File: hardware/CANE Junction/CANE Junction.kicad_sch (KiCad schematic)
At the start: 20 parts, among them J101 Conn_02x05_Odd_Even, SW101 SW_Push, U1 MX25L3233FM2, U101 NCP163ASN330T1G, U102 NCP163ASN330T1G, U103 XMSM0G3507SDGS28R

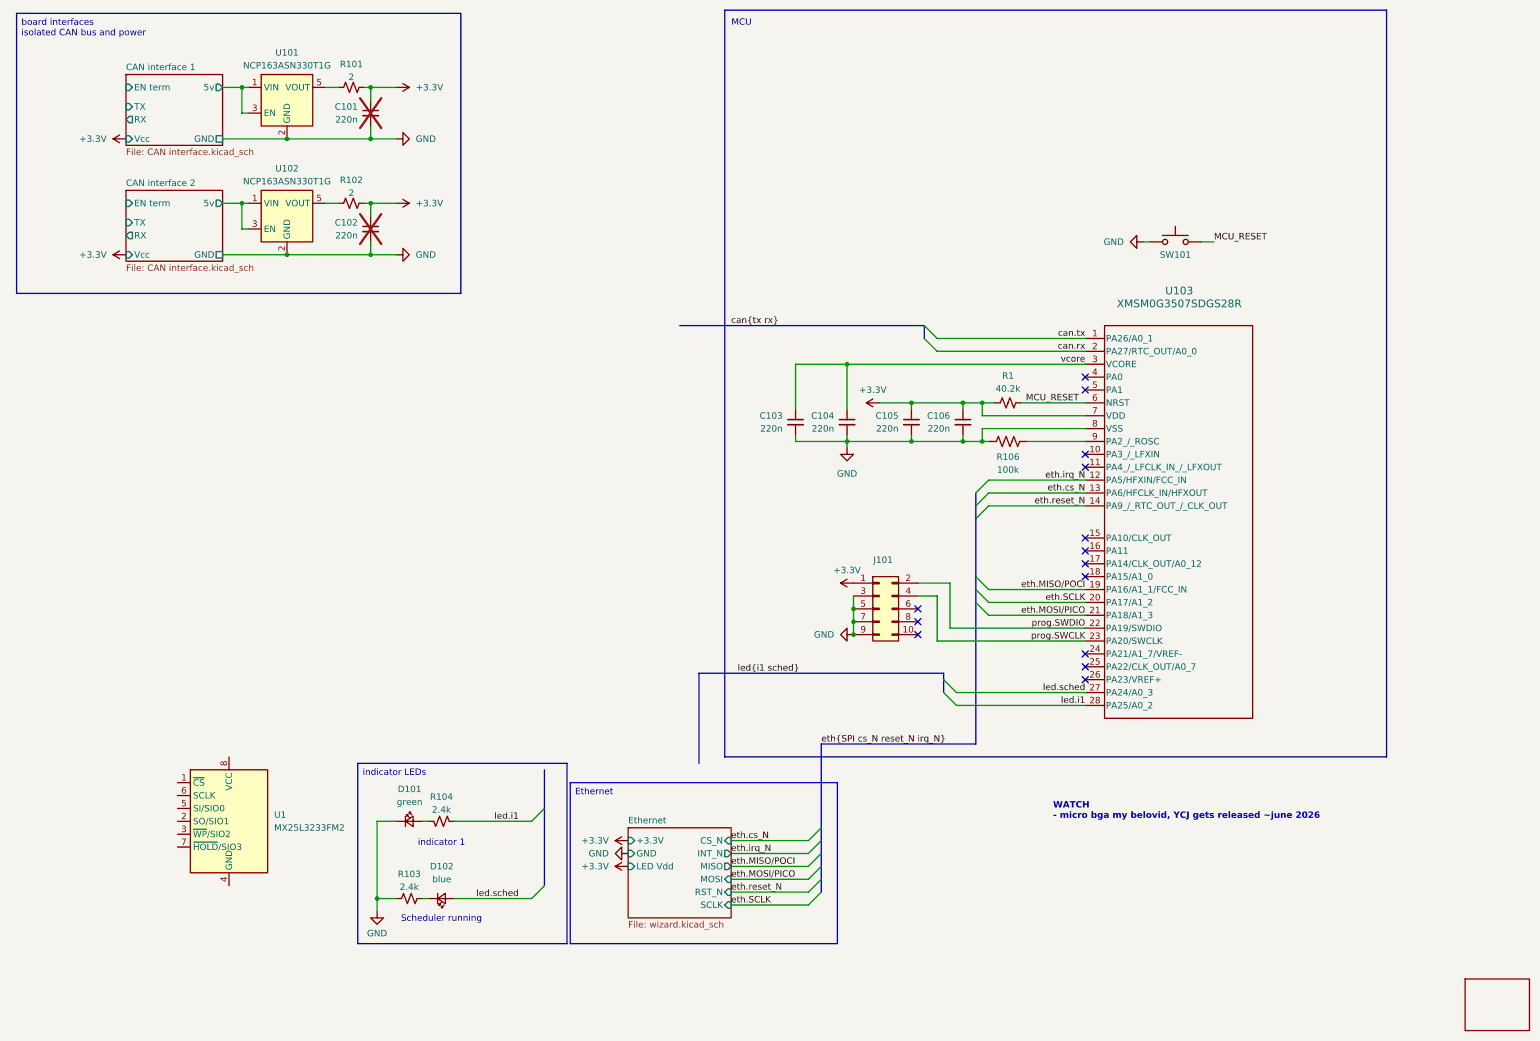
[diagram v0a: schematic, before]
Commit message: shuffle master 2000
nearing terminal shuffle . main components in, awaiting general and layout tie ins
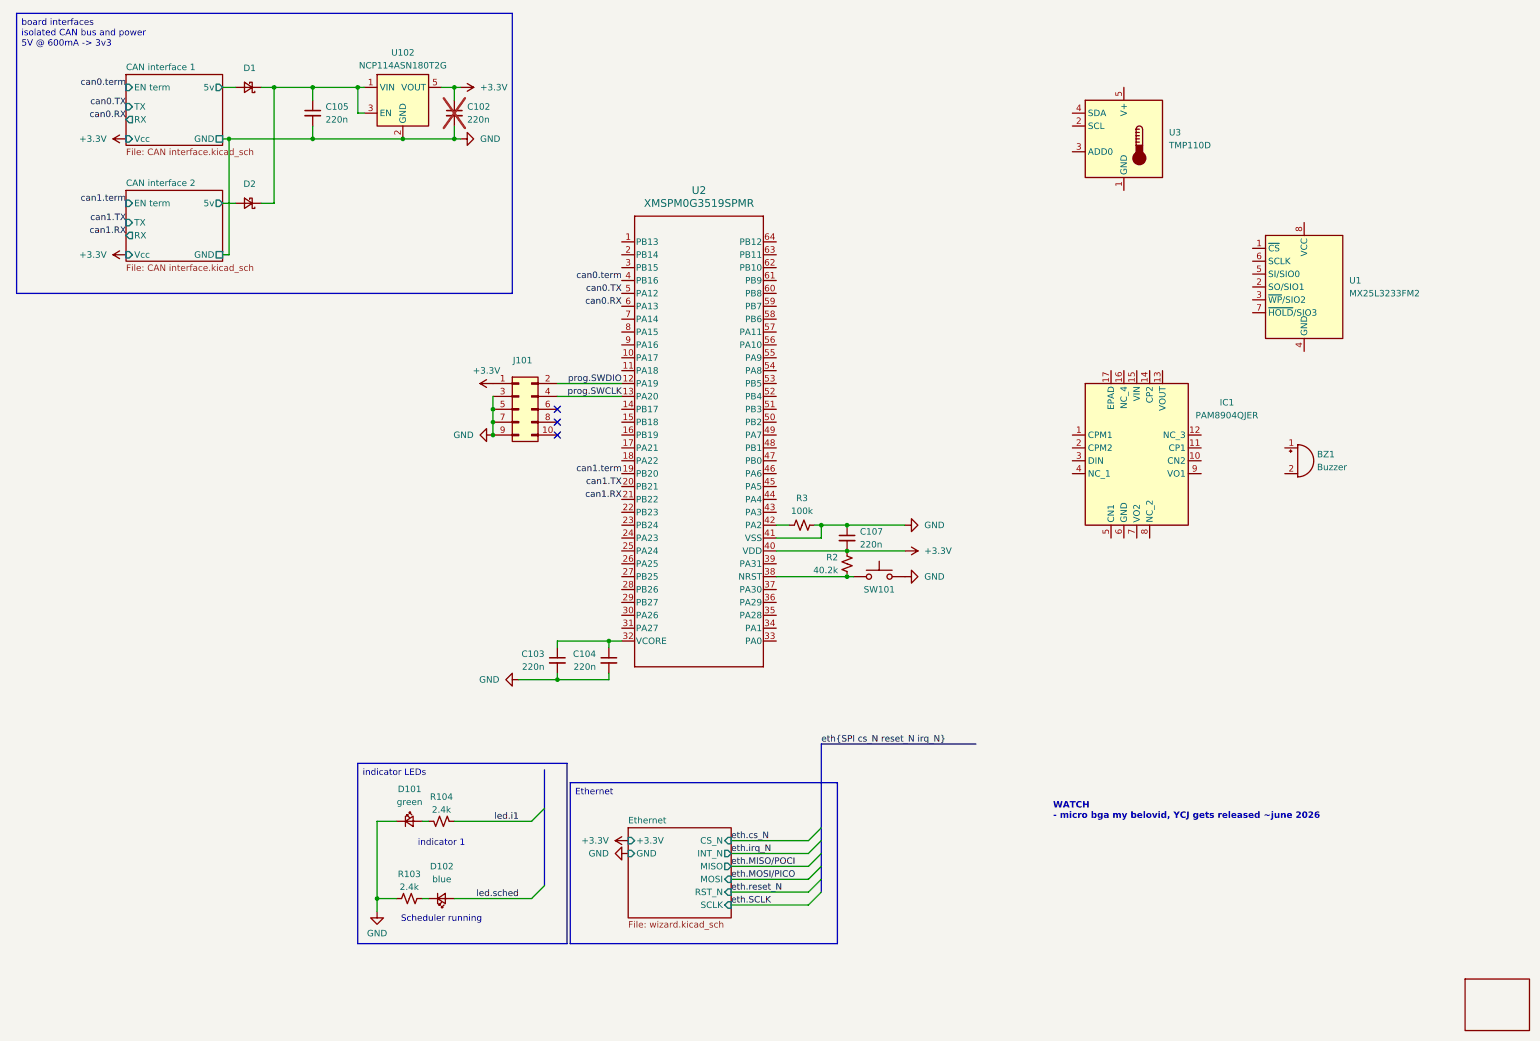
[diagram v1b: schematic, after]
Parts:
- removed C101, C106: 220n, Capacitor_SMD:C_0805_2012Metric_Pad1.18x1.45mm_HandSolder, symbol Device:C_Small
- removed R1: 40.2k, Resistor_SMD:R_0805_2012Metric_Pad1.20x1.40mm_HandSolder, symbol Device:R_Small_US
- removed R101, R102: 2, Resistor_SMD:R_0805_2012Metric_Pad1.20x1.40mm_HandSolder, symbol Device:R_Small_US
- removed R106: 100k, Resistor_SMD:R_1206_3216Metric_Pad1.30x1.75mm_HandSolder, symbol Device:R_US
- removed U101: NCP163ASN330T1G, Package_TO_SOT_SMD:SOT-23-5_HandSoldering, symbol Regulator_Linear:NCP163ASN330T1G
- removed U103: XMSM0G3507SDGS28R, zzLocalLibraries-Footprints:VSSOP28_DGS_TEX-M, symbol zzLocalLibrary:XMSM0G3507SDGS28R
- added BZ1: Buzzer, Buzzer_Beeper:MagneticBuzzer_ProSignal_ABI-009-RC, symbol Device:Buzzer
- added C107: 220n, Capacitor_SMD:C_0805_2012Metric_Pad1.18x1.45mm_HandSolder, symbol Device:C_Small
- added D1, D2: SD0805S020S1R0, Diode_SMD:D_0805_2012Metric_Pad1.15x1.40mm_HandSolder, symbol Device:D_Schottky_Small
- added IC1: PAM8904QJER, zzLocalLibraries-Footprints:QFN50P300X300X65-17N-D, symbol zzLocalLibrary:PAM8904QJER
- added R2: 40.2k, Resistor_SMD:R_0805_2012Metric_Pad1.20x1.40mm_HandSolder, symbol Device:R_Small_US
- added R3: 100k, Resistor_SMD:R_0805_2012Metric_Pad1.20x1.40mm_HandSolder, symbol Device:R_Small_US
- added U2: XMSPM0G3519SPMR, zzLocalLibraries-Footprints:LQFP64_PM_TEX-M, symbol zzLocalLibrary:XMSPM0G3519SPMR
- added U3: TMP110D, Package_SON:Texas_X2SON-5_0.8x0.8mm_P0.48mm_RoutingVia, symbol Sensor_Temperature:TMP110D
- U102: value NCP163ASN330T1G -> NCP114ASN180T2G; mouser https://www.mouser.com/ProductDetail/onsemi/NCP115ASN330T2G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 -> https://www.mouser.com/ProductDetail/onsemi/NCP114ASN180T2G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; note (none) -> careful of built in active discharge
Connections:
- net MCU_RESET is gone; now on net GND: SW101.2
- net +3.3V: now also U102.5 (VOUT), C107.2, R2.1, U2.40 (VDD); no longer C105.1
- net CAN interface 1/5v: now also D1.2 (A)
- net CAN interface 2/5v: now also D2.2 (A); no longer U102.1 (VIN), U102.3 (EN)
- net GND: now also C107.1, R3.1, U2.41 (VSS); no longer SW101.1
- net prog.SWCLK: now also U2.13 (PA20)
- net prog.SWDIO: now also U2.12 (PA19)
- net vcore: no longer names the net of C103.1, C104.1
- net vcore: now also U2.32 (VCORE)
- new net: R2.2, SW101.1, U2.38 (NRST)
- new net: R3.2, U2.42 (PA2)
- new net: C105.1, D1.1 (K), D2.1 (K), U102.1 (VIN), U102.3 (EN)
- new net can0.RX: U2.6 (PA13)
- new net can0.TX: U2.5 (PA12)
- new net can0.term: U2.4 (PB16)
- new net can1.RX: U2.21 (PB22)
- new net can1.TX: U2.20 (PB21)
- new net can1.term: U2.19 (PB20)
- no-connect marks 14 -> 3
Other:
- sheet Ethernet ports: added none; removed LED Vdd
- note removed: "MCU"
- title: BeeMS Master Board (A) -> CANE Junciton
- moved on the sheet: C102, C103, C104, J101, SW101, U1, U102

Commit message: CANE put together and seemingly not exploding
meow meow meow
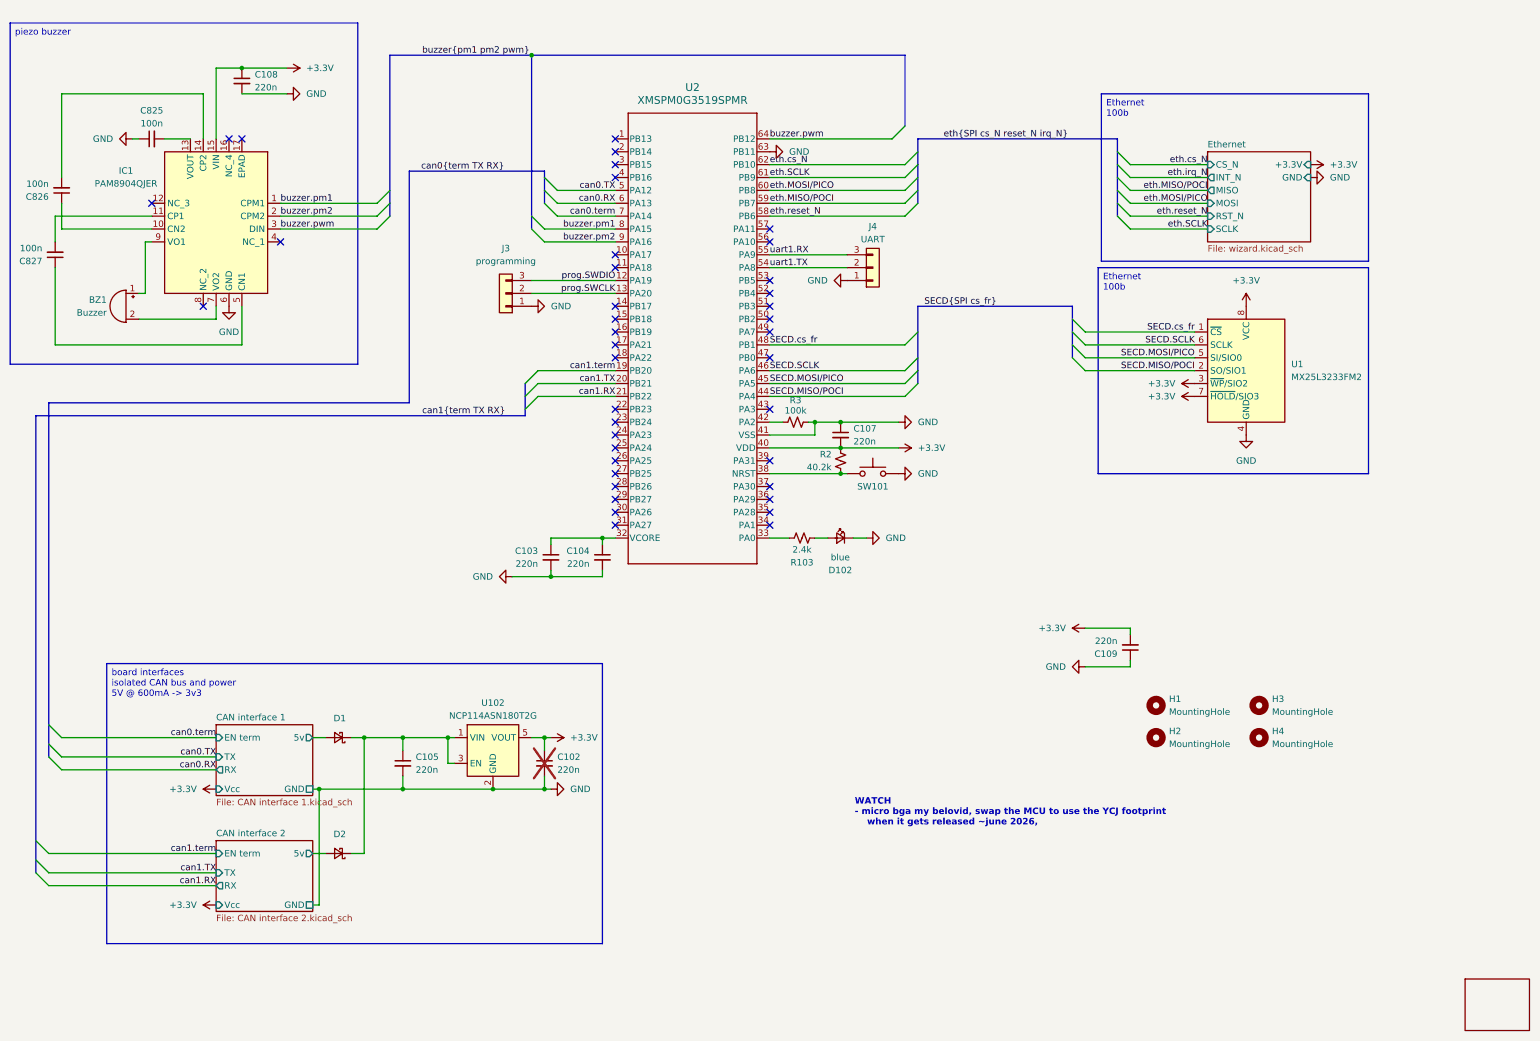
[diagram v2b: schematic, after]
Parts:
- removed D101: green, LED_SMD:LED_0805_2012Metric_Pad1.15x1.40mm_HandSolder, symbol Device:LED_Small
- removed J101: Conn_02x05_Odd_Even, Connector_PinHeader_1.27mm:PinHeader_2x05_P1.27mm_Vertical_SMD, symbol Connector_Generic:Conn_02x05_Odd_Even
- removed R104: 2.4k, Resistor_SMD:R_0805_2012Metric_Pad1.20x1.40mm_HandSolder, symbol Device:R_Small_US
- removed U3: TMP110D, Package_SON:Texas_X2SON-5_0.8x0.8mm_P0.48mm_RoutingVia, symbol Sensor_Temperature:TMP110D
- added C108, C109: 220n, Capacitor_SMD:C_0805_2012Metric_Pad1.18x1.45mm_HandSolder, symbol Device:C_Small
- added C825, C826, C827: 100n, Capacitor_SMD:C_0805_2012Metric_Pad1.18x1.45mm_HandSolder, symbol Device:C_Small
- added H1, H2, H3, H4: MountingHole, MountingHole:MountingHole_4.3mm_M4_ISO7380, symbol Mechanical:MountingHole
- added J3: programming, Connector_PinHeader_2.54mm:PinHeader_1x03_P2.54mm_Vertical, symbol Connector_Generic:Conn_01x03
- added J4: UART, Connector_PinHeader_2.54mm:PinHeader_1x03_P2.54mm_Vertical, symbol Connector_Generic:Conn_01x03
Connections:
- net +3.3V: now also IC1.15 (VIN), U1.3 (~{WP}/SIO2), U1.7 (~{HOLD}/SIO3), U1.8 (VCC), C108.1, C109.2
- net GND: now also D102.1 (K), IC1.6 (GND), U1.4 (GND), U2.63 (PB11), C108.2, C109.1, C825.1, J3.1 (Pin_1), J4.1 (Pin_1); no longer R103.2
- net can0.term: now also U2.7 (PA14); no longer U2.4 (PB16)
- net eth.MISO/POCI: now also U2.59 (PB7)
- net eth.MOSI/PICO: now also U2.60 (PB8)
- net eth.SCLK: now also U2.61 (PB9)
- net eth.cs_N: now also U2.62 (PB10)
- net eth.reset_N: now also U2.58 (PB6)
- net prog.SWCLK: now also J3.2 (Pin_2)
- net prog.SWDIO: now also J3.3 (Pin_3)
- net at U2.33 (PA0): now also R103.1
- net SECD.MISO/POCI: now reaches U2.44 (PA4)
- net SECD.MISO/POCI: now also U1.2 (SO/SIO1)
- net SECD.MOSI/PICO: now reaches U2.45 (PA5)
- net SECD.MOSI/PICO: now also U1.5 (SI/SIO0)
- net SECD.SCLK: now reaches U2.46 (PA6)
- net SECD.SCLK: now also U1.6 (SCLK)
- net SECD.cs_fr: now reaches U2.48 (PB1)
- net SECD.cs_fr: now also U1.1 (~{CS})
- net uart1.TX: now reaches U2.54 (PA8)
- net uart1.TX: now also J4.2 (Pin_2)
- net uart1.RX: now reaches U2.55 (PA9)
- net uart1.RX: now also J4.3 (Pin_3)
- net buzzer.pwm: now reaches U2.64 (PB12)
- net buzzer.pwm: now also IC1.3 (DIN)
- net buzzer.pm1: now reaches U2.8 (PA15)
- net buzzer.pm1: now also IC1.1 (CPM1)
- net buzzer.pm2: now reaches U2.9 (PA16)
- net buzzer.pm2: now also IC1.2 (CPM2)
- net at BZ1.1 (+): now also IC1.9 (VO1)
- net at BZ1.2 (-): now also IC1.7 (VO2)
- net at IC1.10 (CN2): now also C826.1
- net at IC1.11 (CP1): now also C827.2
- net at IC1.13 (VOUT): now also C825.2
- net at IC1.14 (CP2): now also C826.2
- net at IC1.5 (CN1): now also C827.1
- net led.sched: no longer names the net of D102.2 (A)
- net led.sched: now also R103.2
- no-connect marks 3 -> 40
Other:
- sheet CAN interface 1: file CAN interface.kicad_sch -> CAN interface 1.kicad_sch
- sheet CAN interface 2: file CAN interface.kicad_sch -> CAN interface 2.kicad_sch
- note added: "WATCH - micro bga my belovid, swap the MCU to use the YCJ footprint when it gets released ~june 2026,"
- note removed: "Scheduler running"
- note removed: "WATCH - micro bga my belovid, YCJ gets released ~june 2026"
- note removed: "indicator 1"
- moved on the sheet: BZ1, C102, C103, C104, C105, C107, D1, D102, D2, IC1, R103, R2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
